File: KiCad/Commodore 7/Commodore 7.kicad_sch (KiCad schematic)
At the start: 5 parts, among them J1 M20-6112045, U1 IIM-42652 Main Accelerometer, U2 Barometer, U3 IIM-42652 - Main Acceleromete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, U4 BMI270 - Secondary Accelerome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

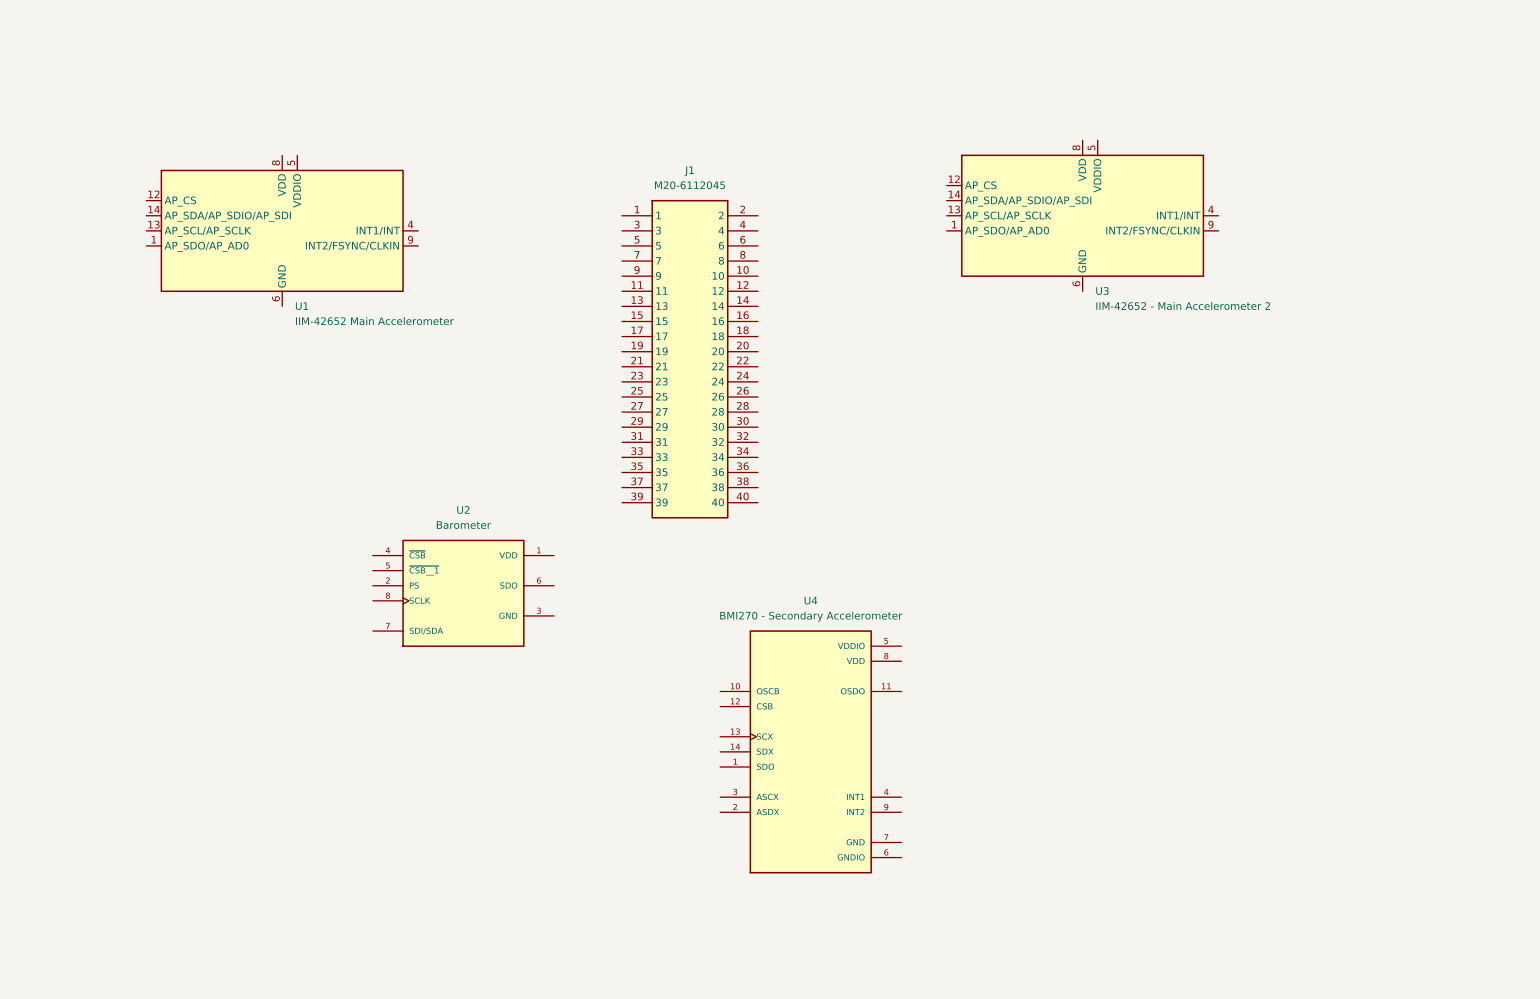
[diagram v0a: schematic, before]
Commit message: hiiiiiiiii!!!!!!!!
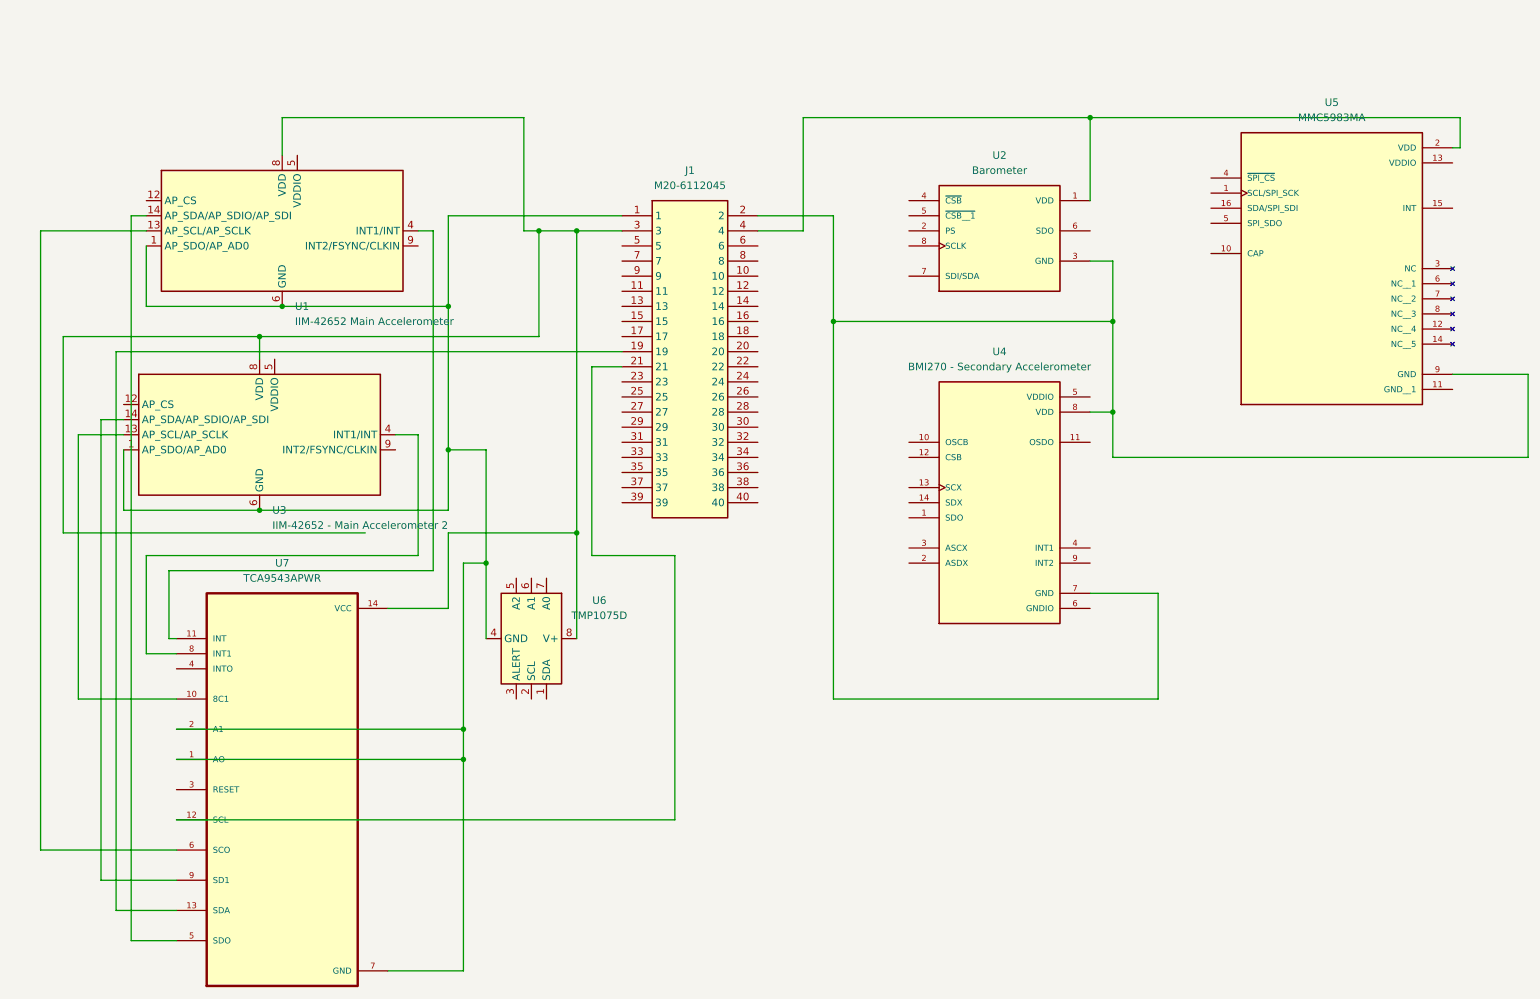
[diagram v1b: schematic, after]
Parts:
- added U5: MMC5983MA, MMC5983MA:PQFN50P300X300X100-16N, symbol MMC5983MA:MMC5983MA
- added U6: TMP1075D, Package_SO:SO-8_3.9x4.9mm_P1.27mm, symbol Sensor_Temperature:TMP1075D
- added U7: TCA9543APWR, TCA9543APWR (1):SOP65P640X120-14N, symbol TCA9543APWR:TCA9543APWR
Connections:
- net at U4.7 (GND): now also J1.2, U2.3 (GND), U4.8 (VDD), U5.9 (GND)
- net at U2.1 (VDD): now also J1.4, U5.2 (VDD)
- net at U3.1 (AP_SDO/AP_AD0): now also J1.1, U1.1 (AP_SDO/AP_AD0), U1.6 (GND), U1.7 (GND), U3.6 (GND), U3.7 (GND), U6.4 (GND), U7.1 (AO), U7.2 (A1), U7.7 (GND)
- net at U3.13 (AP_SCL/AP_SCLK): now also U7.10 (8C1)
- net at U3.14 (AP_SDA/AP_SDIO/AP_SDI): now also U7.9 (SD1)
- net at U3.4 (INT1/INT): now also U7.8 (INT1)
- net at U3.8 (VDD): now also J1.3, U1.8 (VDD), U6.8 (V+), U7.14 (VCC)
- net at U1.13 (AP_SCL/AP_SCLK): now also U7.6 (SCO)
- net at U1.14 (AP_SDA/AP_SDIO/AP_SDI): now also U7.5 (SDO)
- net at U1.4 (INT1/INT): now also U7.11 (INT)
- net at J1.19: now also U7.13 (SDA)
- net at J1.21: now also U7.12 (SCL)
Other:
- moved on the sheet: U2, U3, U4

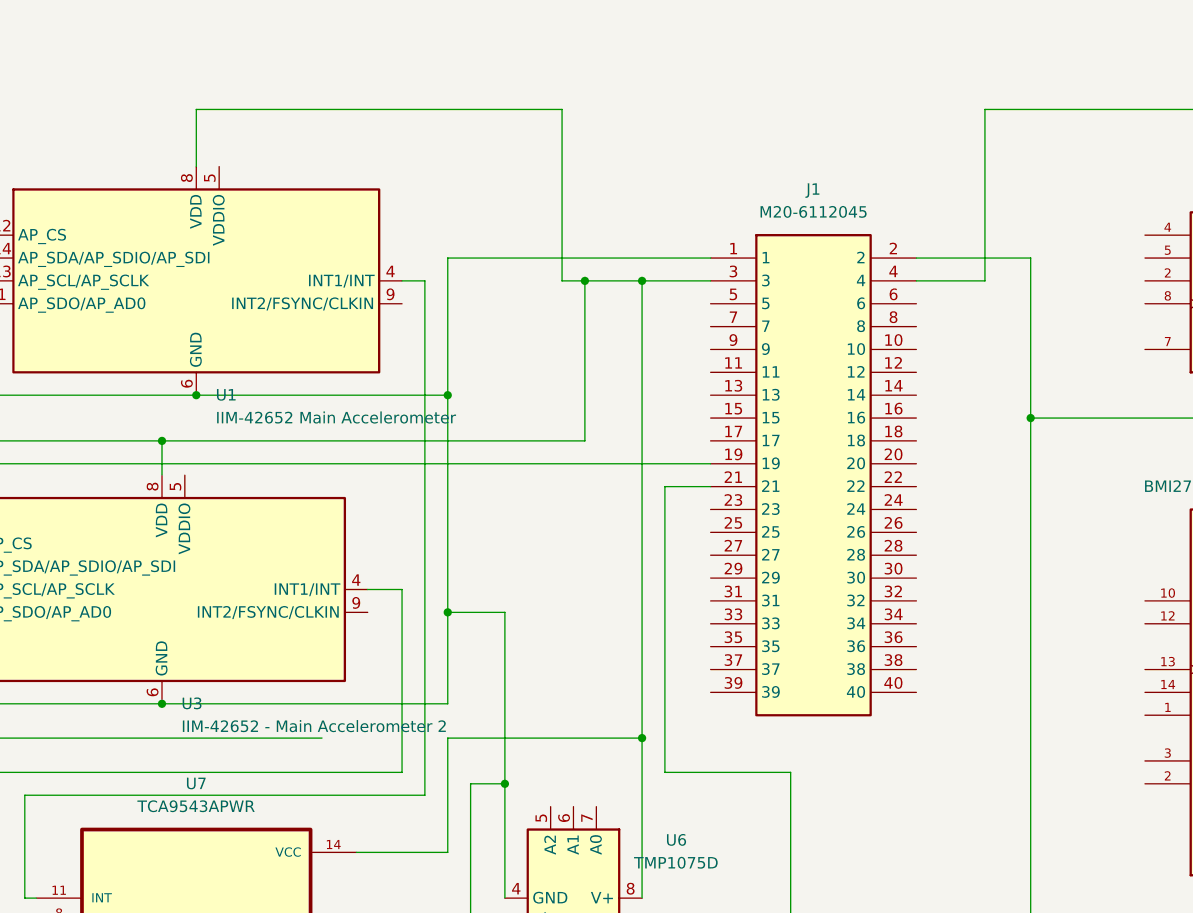
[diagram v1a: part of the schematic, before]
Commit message: heeeloooooooooooo
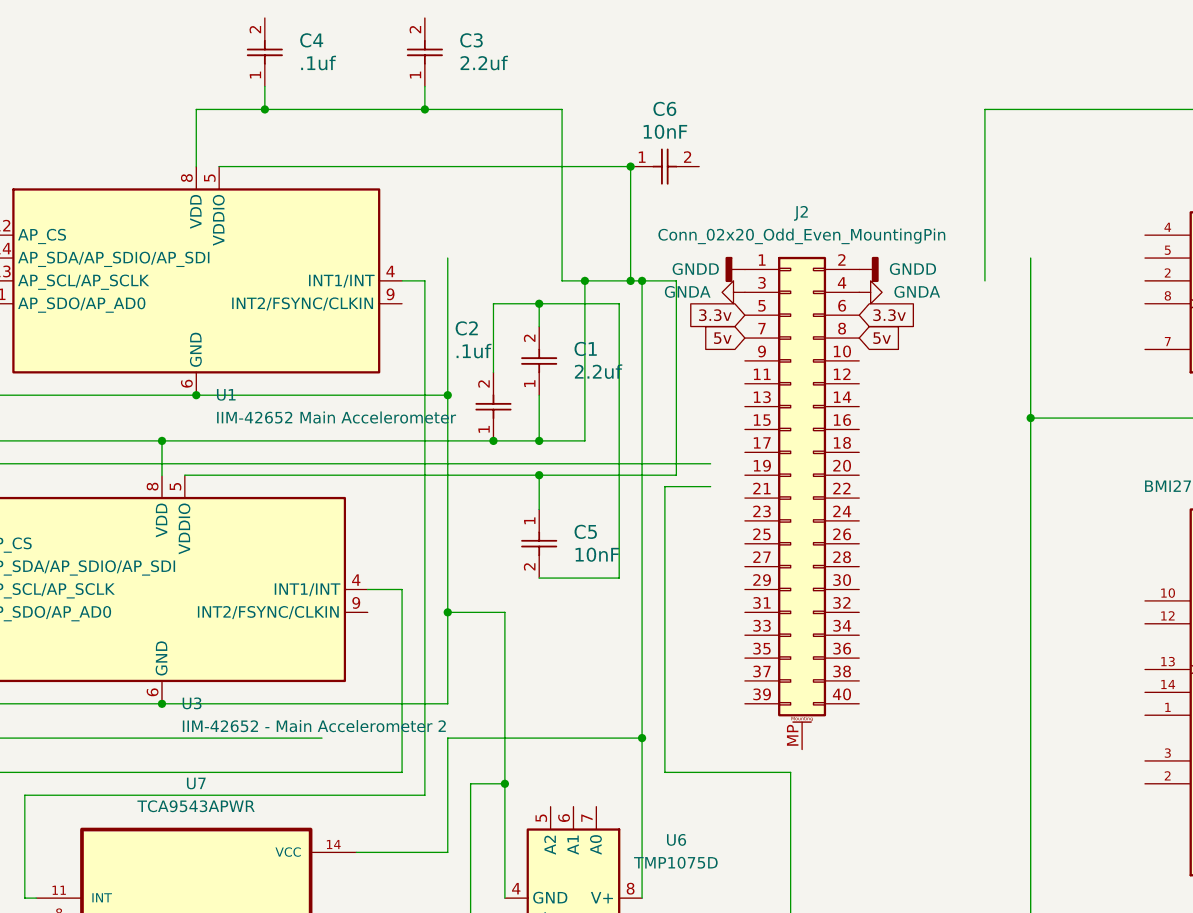
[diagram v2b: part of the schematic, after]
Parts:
- removed J1: M20-6112045, KiCad:RHDR40W69P254_2X20_5146X500X1105P, symbol M20-6112045:M20-6112045
- added C1, C3: 2.2uf, CC0805KK7R7BB225:CAP_CC0805_YAG, symbol 2025-10-06_19-14-39:CC0805KKX7R7BB225
- added C2, C4: .1uf, CC0603KRXQRQBB104:CC0603N_YAG, symbol 2025-10-06_19-12-57:CC0603KRX7R7BB104
- added C5, C6: 10nF, C0603C103K4RECTU:CAPC17595_87N_KEM, symbol 2025-10-06_19-30-10:C0603C103K4RECTU
- added J2: Conn_02x20_Odd_Even_MountingPin, symbol Connector_Generic_MountingPin:Conn_02x20_Odd_Even_MountingPin
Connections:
- net at U1.8 (VDD), U3.8 (VDD), U6.8 (V+)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: now also U1.5 (VDDIO), U3.5 (VDDIO), C1.1, C2.1, C3.1, C4.1, C5.1, C6.1
- new net: C1.2, C2.2, C5.2
- new net 3.3v: J2.5 (Pin_5), J2.6 (Pin_6)
- new net 5v: J2.7 (Pin_7), J2.8 (Pin_8)
- new net GNDA: J2.3 (Pin_3), J2.4 (Pin_4)
- new net GNDD: J2.1 (Pin_1), J2.2 (Pin_2)

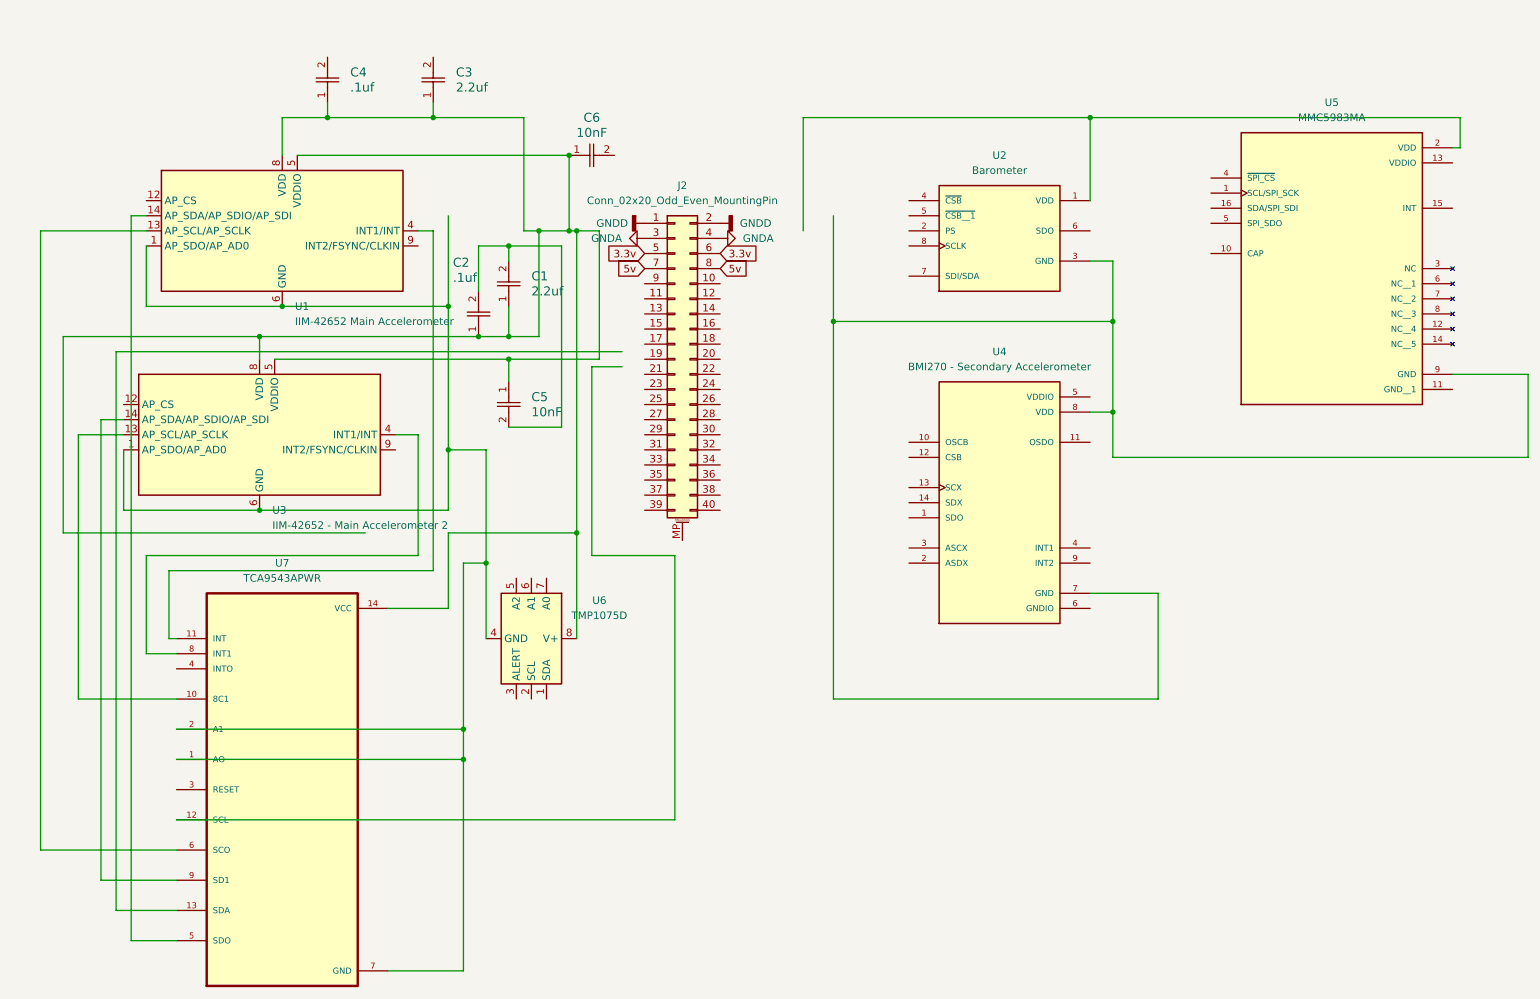
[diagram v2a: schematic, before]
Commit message: oops i delieted everything
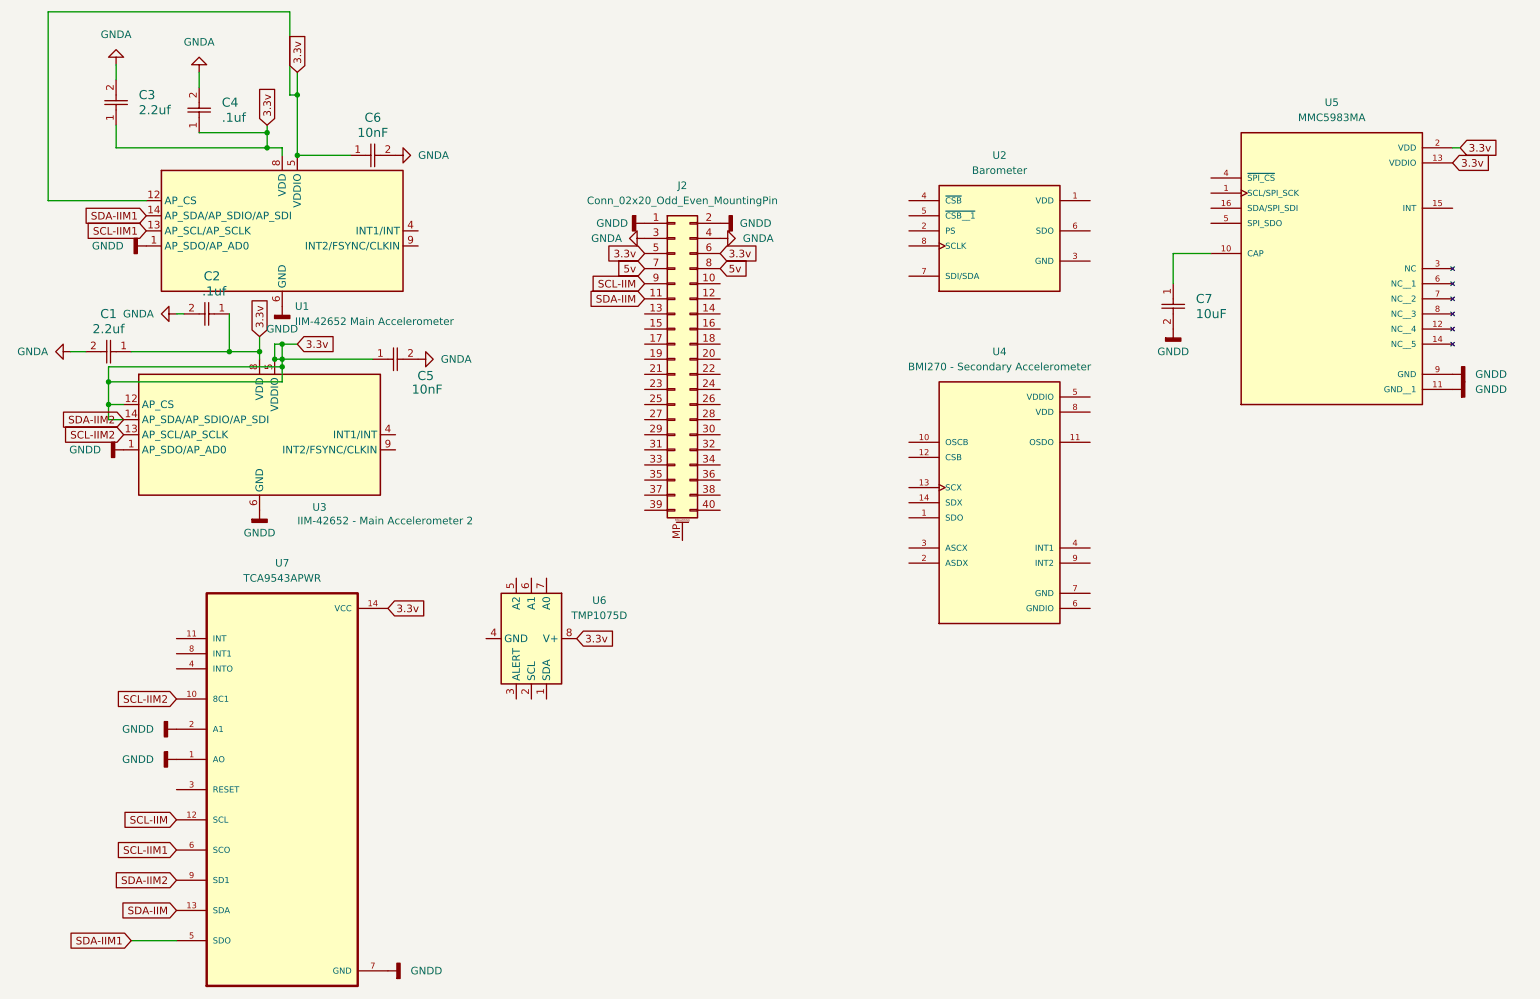
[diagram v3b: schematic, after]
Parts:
- added C7: 10uF, CAPC17595_87N_KEM, symbol 2025-10-06_19-30-10:C0603C103K4RECTU
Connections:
- net 3.3v: now also C1.1, C2.1, C3.1, C4.1, C5.1, C6.1, U1.12 (AP_CS), U1.5 (VDDIO), U1.8 (VDD), U3.12 (AP_CS), U3.14 (AP_SDA/AP_SDIO/AP_SDI), U3.5 (VDDIO), U3.8 (VDD), U5.13 (VDDIO), U5.2 (VDD), U6.8 (V+), U7.14 (VCC), U7.9 (SD1)
- net GNDA: now also C1.2, C2.2, C3.2, C4.2, C5.2, C6.2
- net GNDD: now also U1.1 (AP_SDO/AP_AD0), U1.6 (GND), U1.7 (GND), U3.1 (AP_SDO/AP_AD0), U3.6 (GND), U3.7 (GND), U5.11 (GND__1), U5.9 (GND), U7.1 (AO), U7.2 (A1), U7.7 (GND), C7.2
- net at U5.10 (CAP): now also C7.1
- net at U2.1 (VDD): no longer U5.2 (VDD)
- net SDA-IIM: now reaches J2.11 (Pin_11)
- net SDA-IIM: now also U7.13 (SDA)
- net SCL-IIM: now reaches J2.9 (Pin_9)
- net SCL-IIM: now also U7.12 (SCL)
- net SCL-IIM2: now reaches U3.13 (AP_SCL/AP_SCLK), U7.10 (8C1)
- net at U3.4 (INT1/INT): no longer U7.8 (INT1)
- net SCL-IIM1: now reaches U1.13 (AP_SCL/AP_SCLK), U7.6 (SCO)
- net SDA-IIM1: now reaches U1.14 (AP_SDA/AP_SDIO/AP_SDI), U7.5 (SDO)
- net at U1.4 (INT1/INT): no longer U7.11 (INT)
- now unconnected: U2.3 (GND), U4.7 (GND), U4.8 (VDD), U6.4 (GND)
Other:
- moved on the sheet: C1, C2, C3, C4, C5, C6
